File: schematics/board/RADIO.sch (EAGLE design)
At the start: 47 parts, among them X2 AKKUM

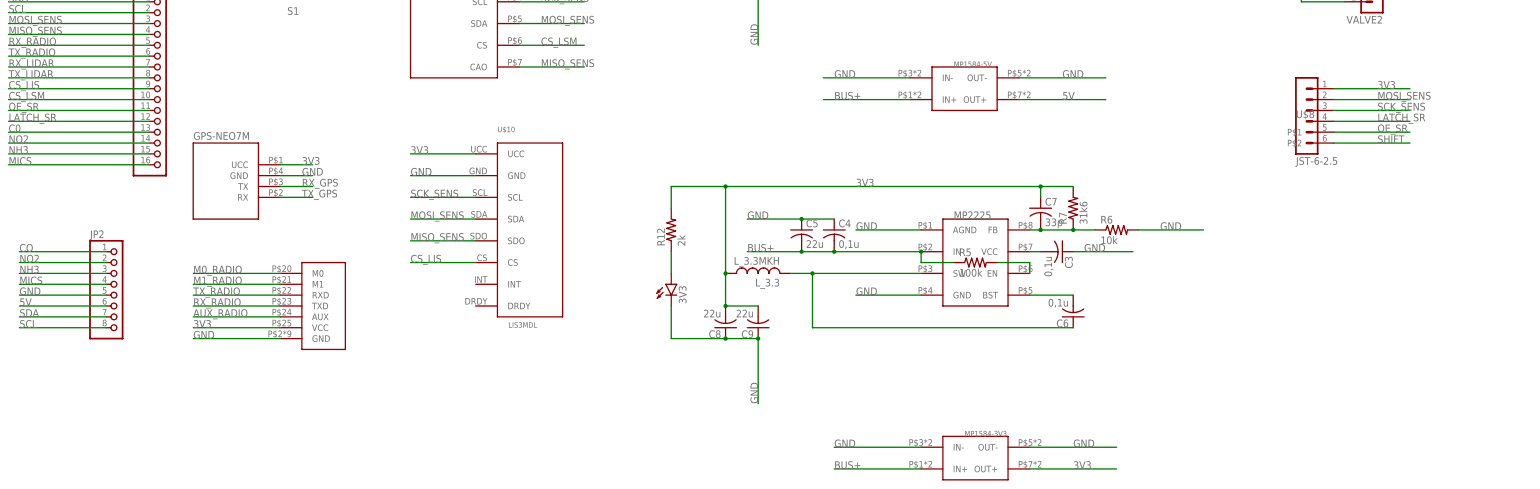
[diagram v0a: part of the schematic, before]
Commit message: Плата Радио
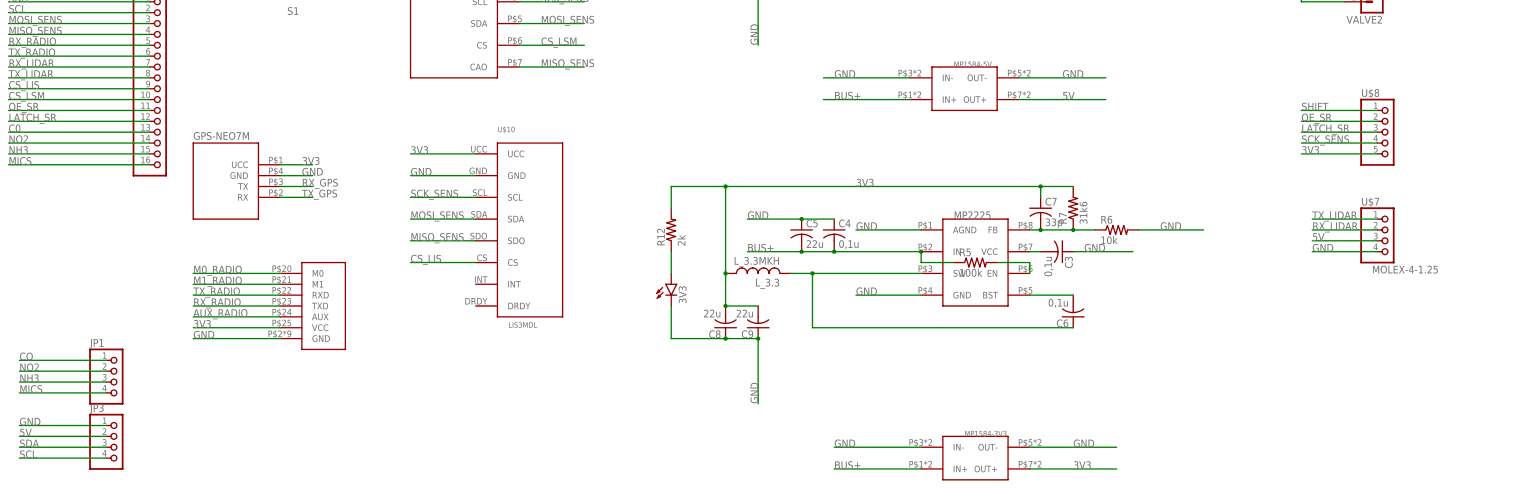
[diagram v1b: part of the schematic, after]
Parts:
- removed JP2: (no value), pinhead:PINHD-1X8
- added JP1, JP3: (no value), pinhead:PINHD-1X4
- added U$7: MOLEX-4-1.25, UNKNOWN-2024:MOLEX-4-1.25
- U$8: value JST-6-2.5 -> MOLEX-5-1.25; device UNKNOWN-2024:JST-6-2.5 -> UNKNOWN-2024:MOLEX-5-1.25
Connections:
- net 3V3: now also U$8.5; no longer U$8.4
- net 5V: now also JP3.2, U$7.3; no longer JP2.6
- net CO: now also JP1.1; no longer JP2.1
- net GND: now also JP3.1, U$7.4; no longer JP2.5
- net LATCH_SR: now also U$8.3; no longer U$8.1
- net MICS: now also JP1.4; no longer JP2.4
- net MOSI_SENS: no longer U$8.3
- net NH3: now also JP1.3; no longer JP2.3
- net NO2: now also JP1.2; no longer JP2.2
- net OE_SR: now also U$8.2; no longer U$8.P$1
- net RX_LIDAR: now also U$7.2
- net SCK_SENS: now also U$8.4; no longer U$8.2
- net SCL: now also JP3.4; no longer JP2.8
- net SDA: now also JP3.3; no longer JP2.7
- net SHIFT: now also U$8.1; no longer U$8.P$2
- net TX_LIDAR: now also U$7.1
